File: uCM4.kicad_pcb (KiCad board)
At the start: 2 copper layers, 55 x 48 mm, 70 parts, among them IC1 MAX17048G+, J10 USB_C_Receptacle, J12 Conn_02x08_Odd_Even, J13 Conn_02x07_Odd_Even, J2 Micro_SD_Card_Det, J4 Conn_01x04, J5 DummyJ, J6 DummyJ, J8 Camera 0, J9 Camera 1, Q2 AO3401A, SW1 SW_DIP_x01, SW3 SW_Push, SW4 SW_SPDT, U1 BNO055, U18 RT9742GGJ5, U2 SN74LVC1G07DBVR, U4 TPS61022, U5 TPD2EUSB30, U6 TP4057

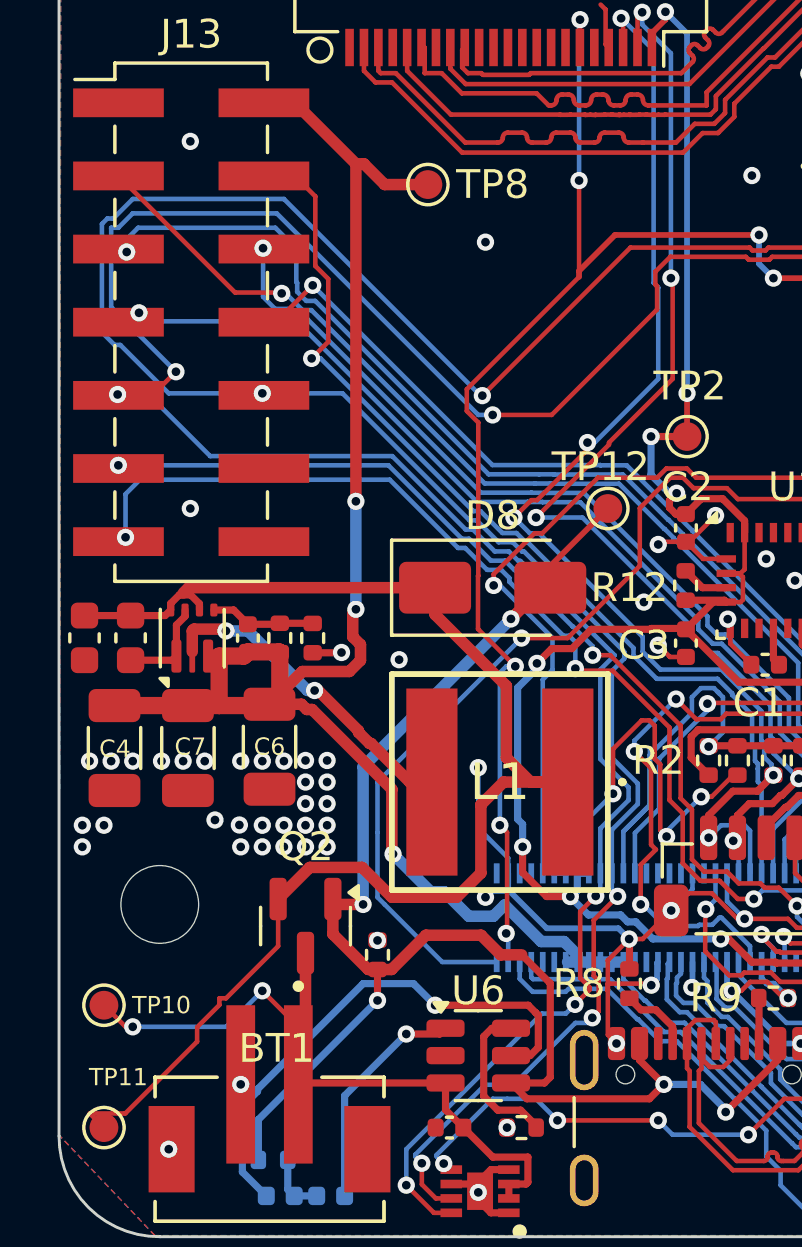
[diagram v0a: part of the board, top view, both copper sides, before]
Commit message: Prepping for production.
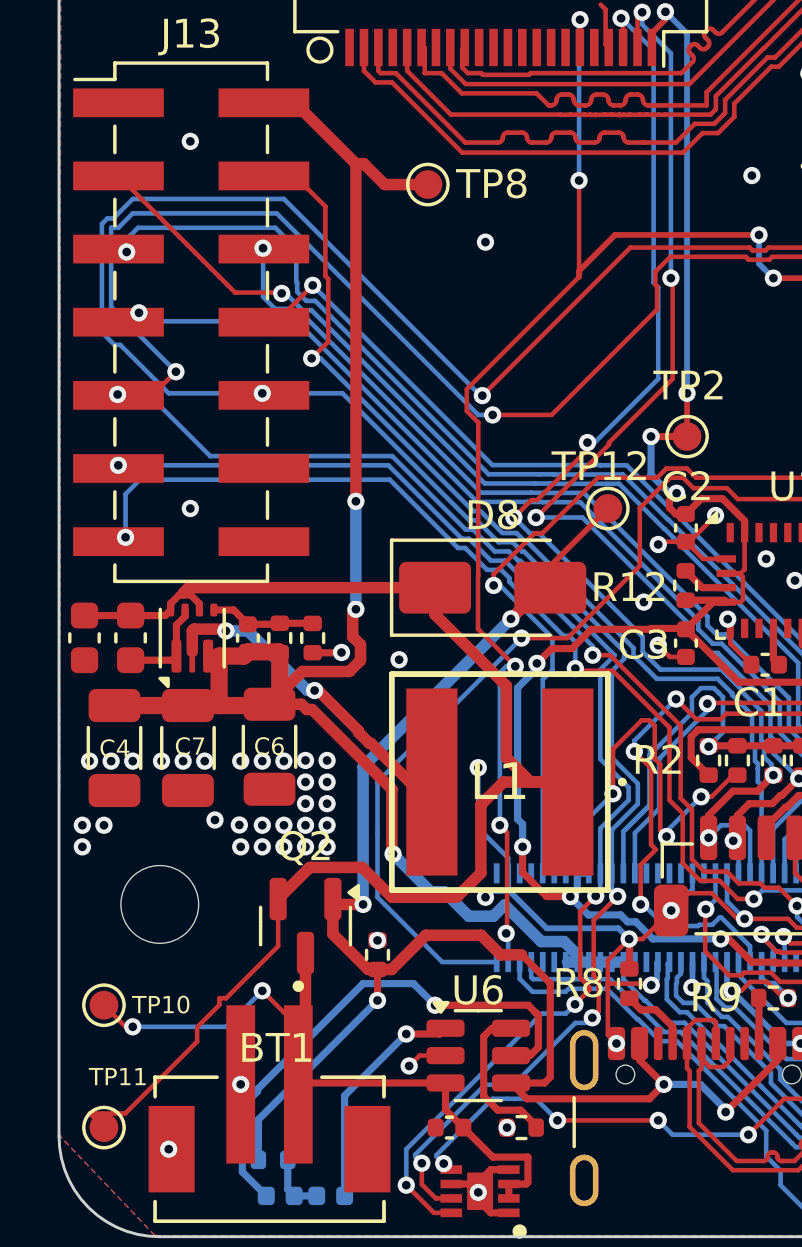
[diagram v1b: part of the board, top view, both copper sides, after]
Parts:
- C5: value 10u -> 10uF
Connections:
- U6 pad 2: unconnected-(U6-GND-Pad2) -> GND
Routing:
- net GND: track 130.3 -> 131.7 mm, vias 93 -> 94
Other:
- board text added: "Shepherd's Eye V1.0 William Nacci Kemere/RNEL + Robinson Labs '25"
